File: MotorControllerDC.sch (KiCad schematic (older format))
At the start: 3 parts

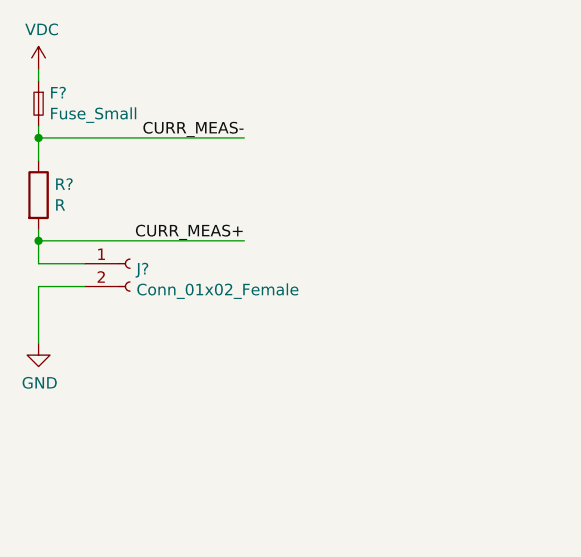
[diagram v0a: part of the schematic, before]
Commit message: Simulation in progress
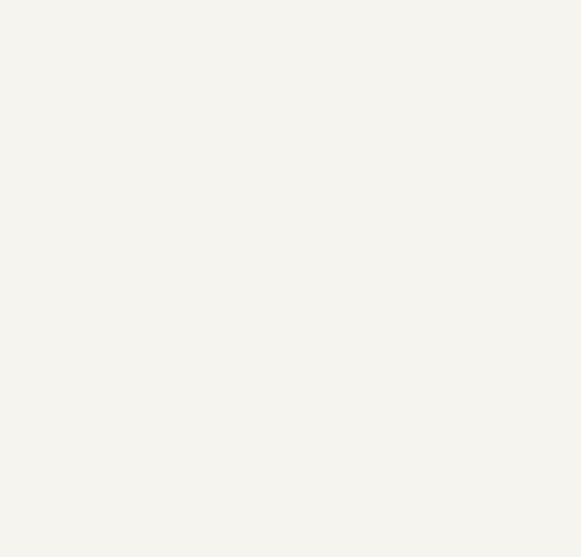
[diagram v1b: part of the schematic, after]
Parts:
- removed F?: Fuse_Small, symbol Device:Fuse_Small
- removed J?: Conn_01x02_Female, symbol Connector:Conn_01x02_Female
- removed R?: R, symbol Device:R
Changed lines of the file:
@@
 Text Notes 7100 7000 0    50   ~ 0
 Designed By: Jaden Bottemiller
-$Comp
-L Connector:Conn_01x02_Female J?
-U 1 1 5E605EB6
-P 1050 1550
-F 0 "J?" H 1078 1526 50  0000 L CNN
-F 1 "Conn_01x02_Female" H 1078 1435 50  0000 L CNN
-F 2 "" H 1050 1550 50  0001 C CNN
-F 3 "~" H 1050 1550 50  0001 C CNN
-	1    1050 1550
-	1    0    0    -1
-$EndComp
-Wire Wire Line
-	850  1650 650  1650
-Wire Wire Line
-	650  1650 650  1900
-$Comp
-L power:GND #PWR?
-U 1 1 5E607E1E
-P 650 1900
-F 0 "#PWR?" H 650 1650 50  0001 C CNN
-F 1 "GND" H 655 1727 50  0000 C CNN
-F 2 "" H 650 1900 50  0001 C CNN
-F 3 "" H 650 1900 50  0001 C CNN
-	1    650  1900
-	1    0    0    -1
-$EndComp
-$Comp
-L Device:Fuse_Small F?
-U 1 1 5E60B316
-P 650 850
-F 0 "F?" V 604 898 50  0000 L CNN
-F 1 "Fuse_Small" V 695 898 50  0000 L CNN
-F 2 "" H 650 850 50  0001 C CNN
-F 3 "~" H 650 850 50  0001 C CNN
-	1    650  850
-	0    1    1    0
-$EndComp
-Wire Wire Line
-	650  1550 850  1550
-Wire Wire Line
-	650  750  650  700
-$Comp
-L power:VDC #PWR?
-U 1 1 5E60D008
-P 650 700
-F 0 "#PWR?" H 650 600 50  0001 C CNN
-F 1 "VDC" H 665 873 50  0000 C CNN
-F 2 "" H 650 700 50  0001 C CNN
-F 3 "" H 650 700 50  0001 C CNN
-	1    650  700
-	1    0    0    -1
-$EndComp
-$Comp
-L Device:R R?
-U 1 1 5E610D8D
-P 650 1250
-F 0 "R?" H 720 1296 50  0000 L CNN
-F 1 "R" H 720 1205 50  0000 L CNN
-F 2 "" V 580 1250 50  0001 C CNN
-F 3 "~" H 650 1250 50  0001 C CNN
-	1    650  1250
-	1    0    0    -1
-$EndComp
-Wire Wire Line
-	650  1550 650  1450
-Wire Wire Line
-	650  1100 650  1000
-Wire Wire Line
-	650  1450 1550 1450
-Connection ~ 650  1450
-Wire Wire Line
-	650  1450 650  1400
-Wire Wire Line
-	650  1000 1550 1000
-Connection ~ 650  1000
-Wire Wire Line
-	650  1000 650  950
-Text Label 1550 1000 2    50   ~ 0
-CURR_MEAS-
-Text Label 1550 1450 2    50   ~ 0
-CURR_MEAS+
 $EndSCHEMATC

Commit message: Added randoms stuff
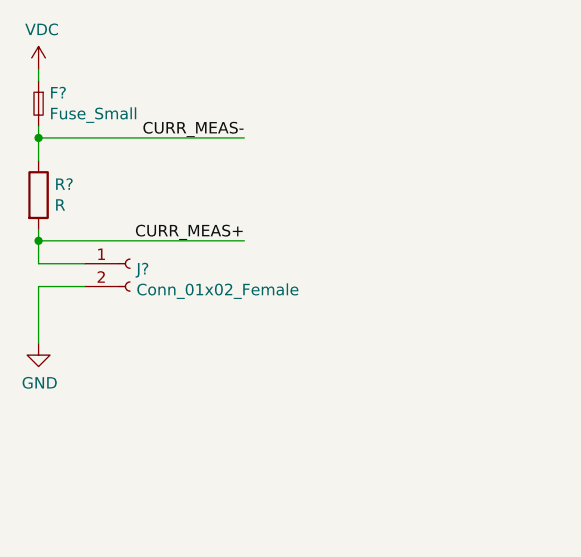
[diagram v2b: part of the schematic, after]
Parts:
- added F?: Fuse_Small, symbol Device:Fuse_Small
- added J?: Conn_01x02_Female, symbol Connector:Conn_01x02_Female
- added R?: R, symbol Device:R
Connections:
- new net CURR_MEAS+: J?.1 (Pin_1), R?.2
- new net CURR_MEAS-: F?.2, R?.1
- new net GND: J?.2 (Pin_2)
- new net VDC: F?.1
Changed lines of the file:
@@
 Text Notes 7100 7000 0    50   ~ 0
 Designed By: Jaden Bottemiller
+$Comp
+L Connector:Conn_01x02_Female J?
+U 1 1 5E605EB6
+P 1050 1550
+F 0 "J?" H 1078 1526 50  0000 L CNN
+F 1 "Conn_01x02_Female" H 1078 1435 50  0000 L CNN
+F 2 "" H 1050 1550 50  0001 C CNN
+F 3 "~" H 1050 1550 50  0001 C CNN
+	1    1050 1550
+	1    0    0    -1
+$EndComp
+Wire Wire Line
+	850  1650 650  1650
+Wire Wire Line
+	650  1650 650  1900
+$Comp
+L power:GND #PWR?
+U 1 1 5E607E1E
+P 650 1900
+F 0 "#PWR?" H 650 1650 50  0001 C CNN
+F 1 "GND" H 655 1727 50  0000 C CNN
+F 2 "" H 650 1900 50  0001 C CNN
+F 3 "" H 650 1900 50  0001 C CNN
+	1    650  1900
+	1    0    0    -1
+$EndComp
+$Comp
+L Device:Fuse_Small F?
+U 1 1 5E60B316
+P 650 850
+F 0 "F?" V 604 898 50  0000 L CNN
+F 1 "Fuse_Small" V 695 898 50  0000 L CNN
+F 2 "" H 650 850 50  0001 C CNN
+F 3 "~" H 650 850 50  0001 C CNN
+	1    650  850
+	0    1    1    0
+$EndComp
+Wire Wire Line
+	650  1550 850  1550
+Wire Wire Line
+	650  750  650  700
+$Comp
+L power:VDC #PWR?
+U 1 1 5E60D008
+P 650 700
+F 0 "#PWR?" H 650 600 50  0001 C CNN
+F 1 "VDC" H 665 873 50  0000 C CNN
+F 2 "" H 650 700 50  0001 C CNN
+F 3 "" H 650 700 50  0001 C CNN
+	1    650  700
+	1    0    0    -1
+$EndComp
+$Comp
+L Device:R R?
+U 1 1 5E610D8D
+P 650 1250
+F 0 "R?" H 720 1296 50  0000 L CNN
+F 1 "R" H 720 1205 50  0000 L CNN
+F 2 "" V 580 1250 50  0001 C CNN
+F 3 "~" H 650 1250 50  0001 C CNN
+	1    650  1250
+	1    0    0    -1
+$EndComp
+Wire Wire Line
+	650  1550 650  1450
+Wire Wire Line
+	650  1100 650  1000
+Wire Wire Line
+	650  1450 1550 1450
+Connection ~ 650  1450
+Wire Wire Line
+	650  1450 650  1400
+Wire Wire Line
+	650  1000 1550 1000
+Connection ~ 650  1000
+Wire Wire Line
+	650  1000 650  950
+Text Label 1550 1000 2    50   ~ 0
+CURR_MEAS-
+Text Label 1550 1450 2    50   ~ 0
+CURR_MEAS+
 $EndSCHEMATC
